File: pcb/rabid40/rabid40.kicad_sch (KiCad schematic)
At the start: 136 parts, among them J1 SWD, J2 Conn_01x04, J3 MX_SW_solder, K1 MX_SW_solder, M1 MX_SW_solder, P1 MX_SW_solder, Q1 MX_SW_solder, SW7 SW_Push, T1 MX_SW_solder, U1 RP2040, U2 W25Q128JVS, U3 XC6206PxxxMR-Regulator_Linear, U4 MX_SW_solder, X1 MX_SW_solder, Y1 12MHz, Y2 MX_SW_solder

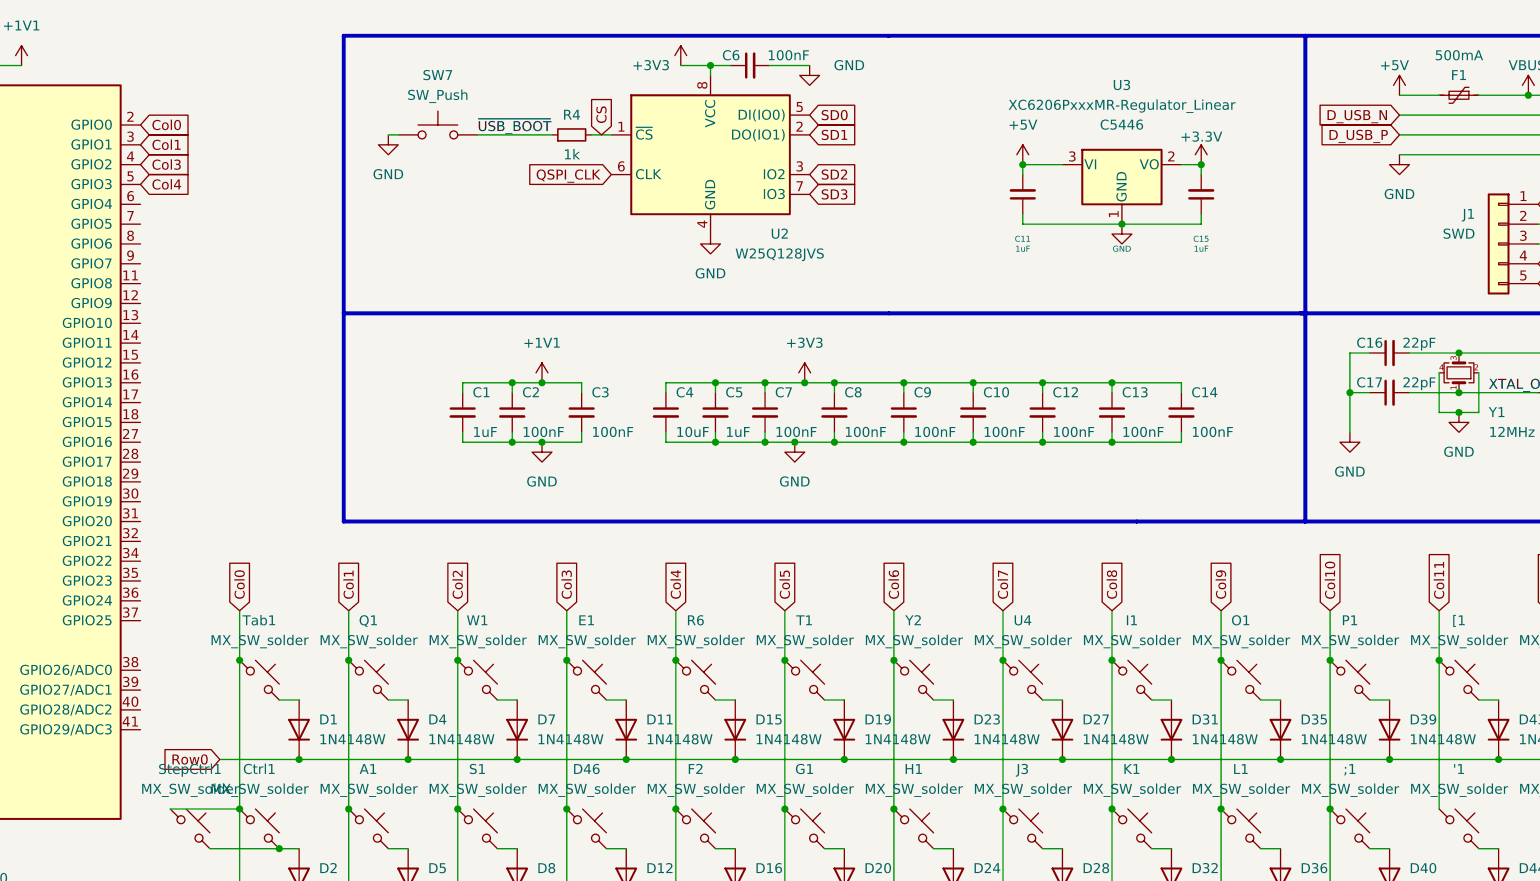
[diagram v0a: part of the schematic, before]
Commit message: completed routing
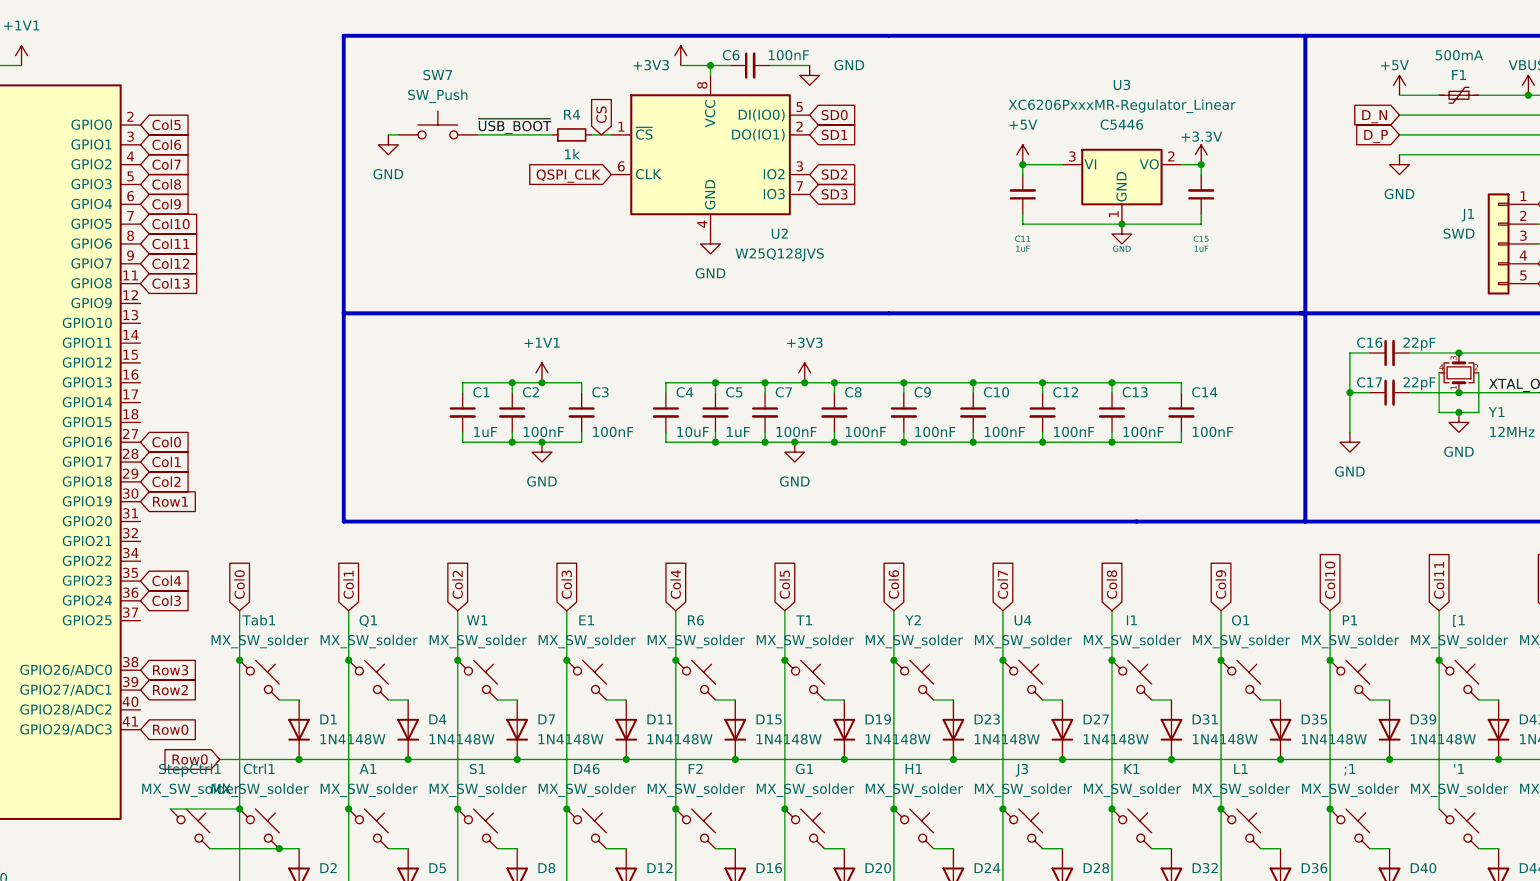
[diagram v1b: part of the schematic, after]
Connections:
- net D_USB_N is gone; now on net D_N: J2.2 (Pin_2)
- net D_USB_P is gone; now on net D_P: J2.3 (Pin_3)
- net Col0: now also U1.27 (GPIO16); no longer U1.2 (GPIO0)
- net Col1: now also U1.28 (GPIO17); no longer U1.3 (GPIO1)
- net Col10: now also U1.7 (GPIO5)
- net Col11: now also U1.8 (GPIO6)
- net Col12: now also U1.9 (GPIO7)
- net Col13: now also U1.11 (GPIO8)
- net Col2: now also U1.29 (GPIO18)
- net Col3: now also U1.36 (GPIO24); no longer U1.4 (GPIO2)
- net Col4: now also U1.35 (GPIO23); no longer U1.5 (GPIO3)
- net Col5: now also U1.2 (GPIO0)
- net Col6: now also U1.3 (GPIO1)
- net Col7: now also U1.4 (GPIO2)
- net Col8: now also U1.5 (GPIO3)
- net Col9: now also U1.6 (GPIO4)
- net Row0: now also U1.41 (GPIO29/ADC3)
- net Row1: now also U1.30 (GPIO19)
- net Row2: now also U1.39 (GPIO27/ADC1)
- net Row3: now also U1.38 (GPIO26/ADC0)
